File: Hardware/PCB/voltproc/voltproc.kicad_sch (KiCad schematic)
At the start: 15 parts, among them J1 Synth_power_2x5, J2 2_pin_Molex_header, J3 2_pin_Molex_header, J4 Conn_01x13, J5 2_pin_Molex_connector, J6 2_pin_Molex_connector, J7 Conn_01x13

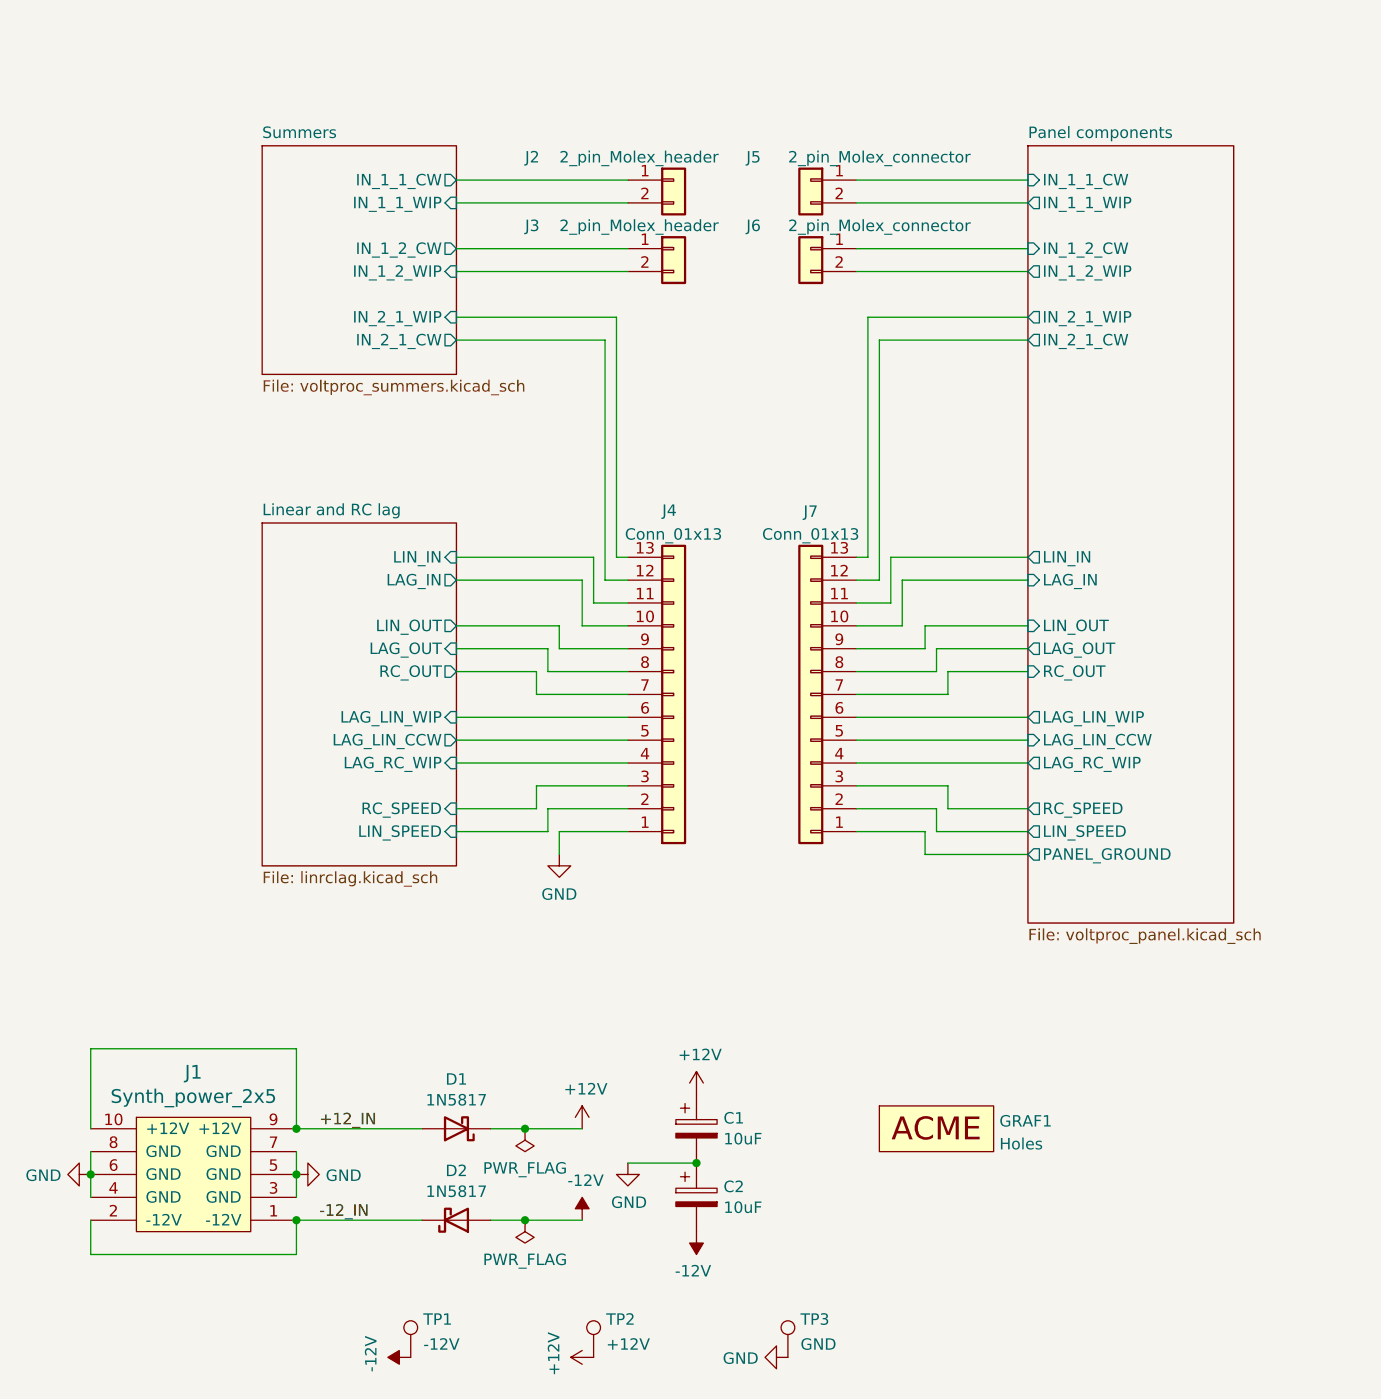
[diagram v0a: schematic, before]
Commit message: post breadboard revisions
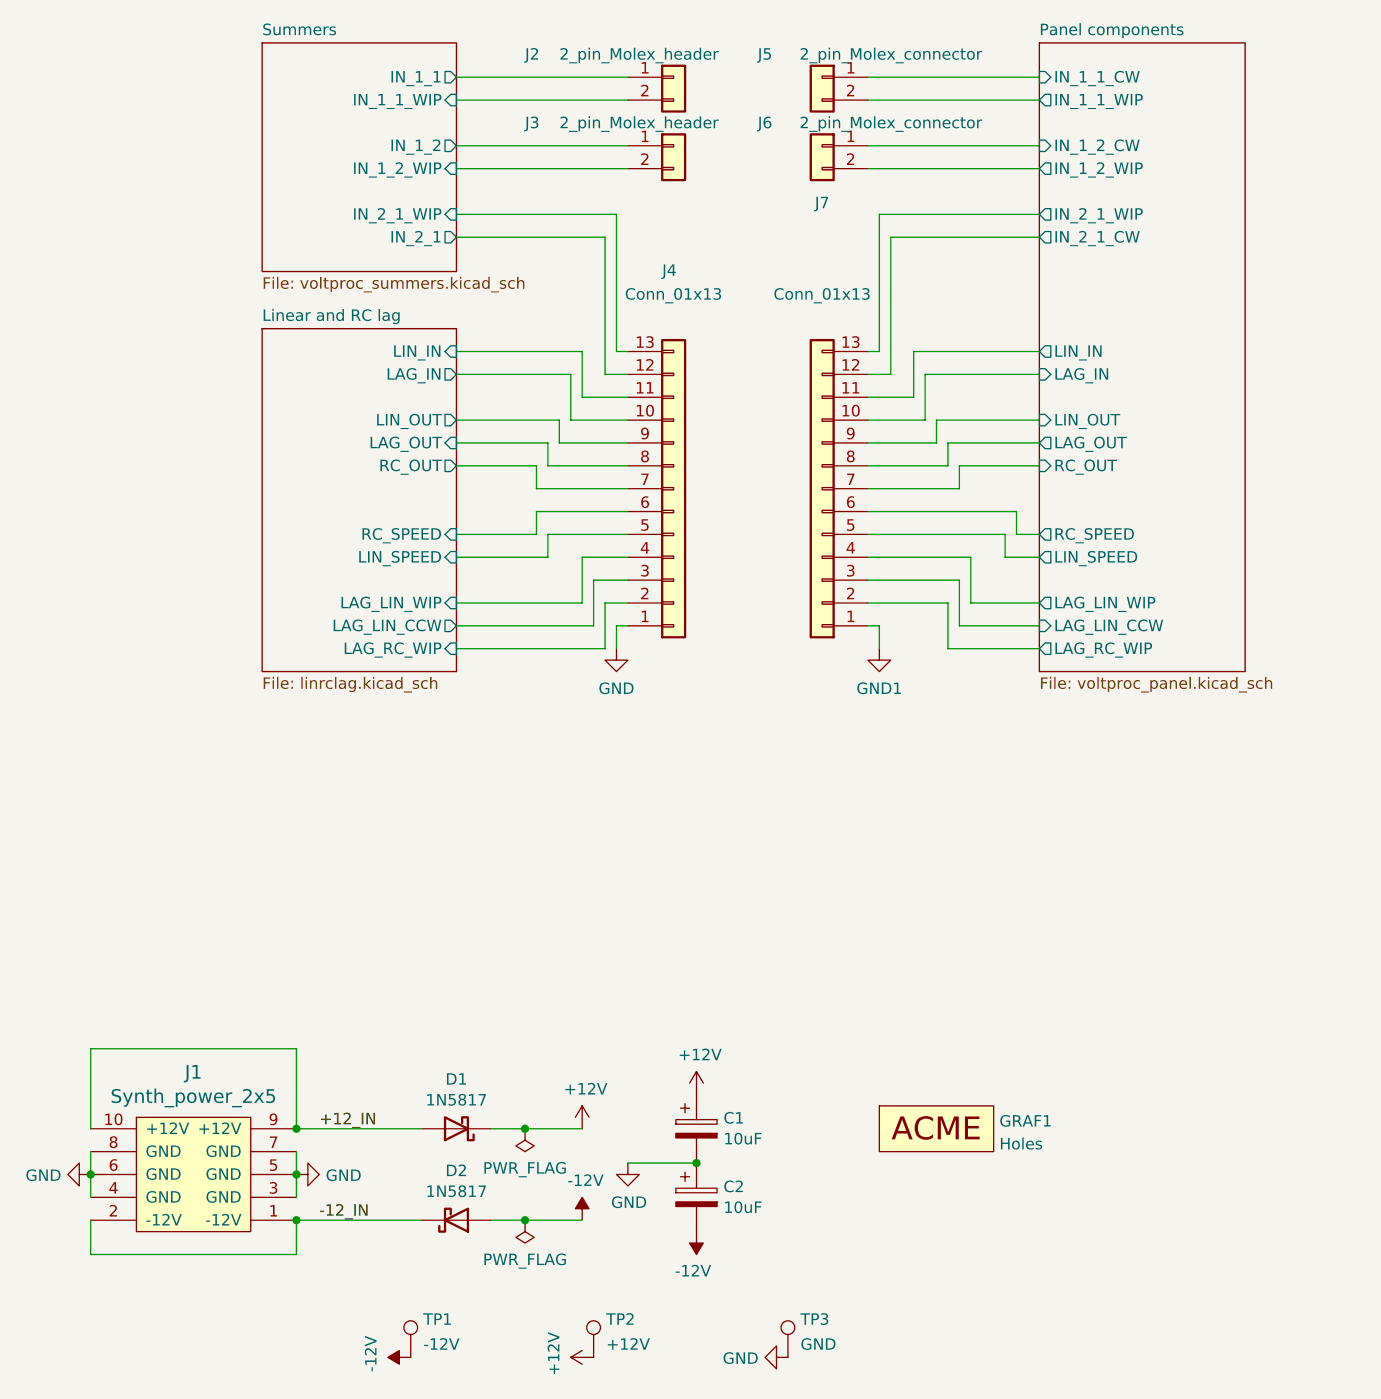
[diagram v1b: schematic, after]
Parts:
- TP1, TP2: Config (none) -> DNF; now left out of the parts list
- TP3: footprint ao_tht:TestPoint_THTPad_1.5x1.5mm_Drill0.7mm -> ao_tht:TestPoint_THTPad_D1.5mm_Drill0.7mm; Config (none) -> DNF; now left out of the parts list
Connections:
- net Linear and RC lag/LAG_LIN_CCW: now also J4.3 (Pin_3); no longer J4.5 (Pin_5)
- net Linear and RC lag/LAG_LIN_WIP: now also J4.4 (Pin_4); no longer J4.6 (Pin_6)
- net Linear and RC lag/LAG_RC_WIP: now also J4.2 (Pin_2); no longer J4.4 (Pin_4)
- net Linear and RC lag/LIN_SPEED: now also J4.5 (Pin_5); no longer J4.2 (Pin_2)
- net Linear and RC lag/RC_SPEED: now also J4.6 (Pin_6); no longer J4.3 (Pin_3)
- net Panel components/LAG_LIN_CCW: now also J7.3 (Pin_3); no longer J7.5 (Pin_5)
- net Panel components/LAG_LIN_WIP: now also J7.4 (Pin_4); no longer J7.6 (Pin_6)
- net Panel components/LAG_RC_WIP: now also J7.2 (Pin_2); no longer J7.4 (Pin_4)
- net Panel components/LIN_SPEED: now also J7.5 (Pin_5); no longer J7.2 (Pin_2)
- net Panel components/RC_SPEED: now also J7.6 (Pin_6); no longer J7.3 (Pin_3)
- net Panel components/PANEL_GROUND renamed GND1
- net Summers/IN_1_1_CW renamed Summers/IN_1_1
- net Summers/IN_1_2_CW renamed Summers/IN_1_2
- net Summers/IN_2_1_CW renamed Summers/IN_2_1
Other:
- sheet Panel components ports: added none; removed PANEL_GROUND
- sheet Summers ports: added IN_1_1, IN_1_2, IN_2_1; removed IN_1_1_CW, IN_1_2_CW, IN_2_1_CW
- moved on the sheet: J2, J3, J4, J5, J6, J7
